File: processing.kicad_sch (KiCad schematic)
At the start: 29 parts, among them U2 DLF162500LT-5028A1, U6 STM32WB35C_C-E_UxA, Y1 32MHz, Y2 32kHz

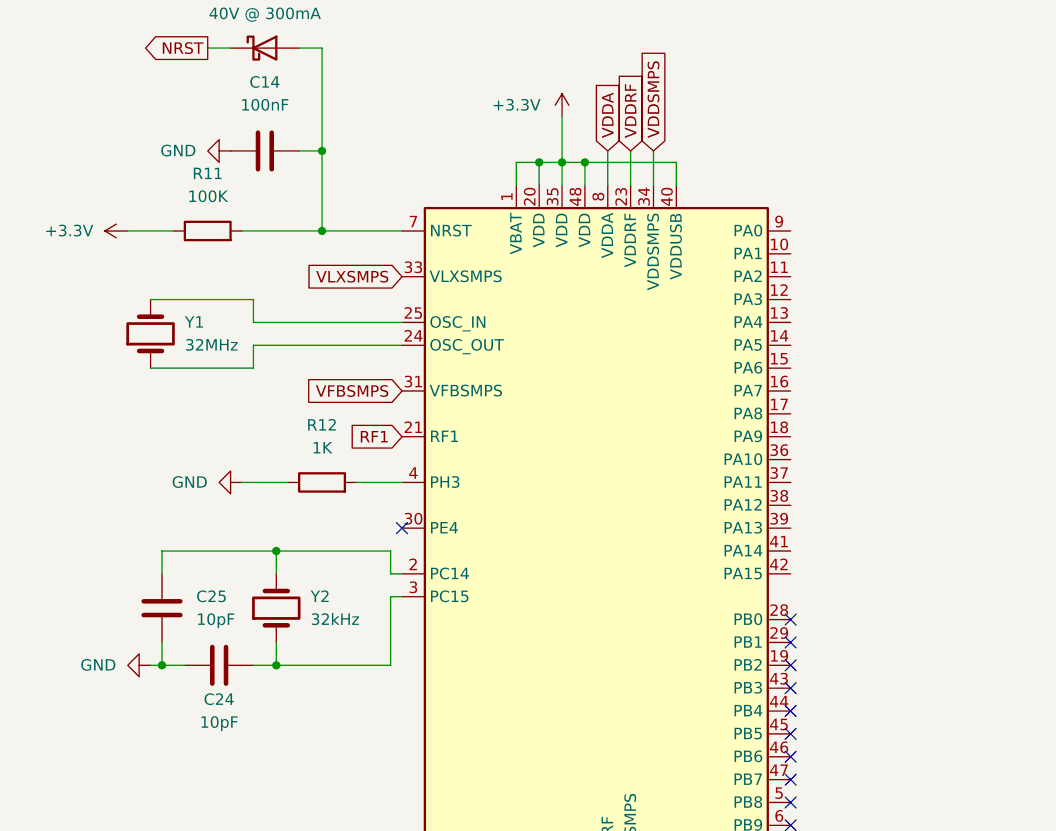
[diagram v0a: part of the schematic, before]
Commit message: Catalogued in raja.rocks
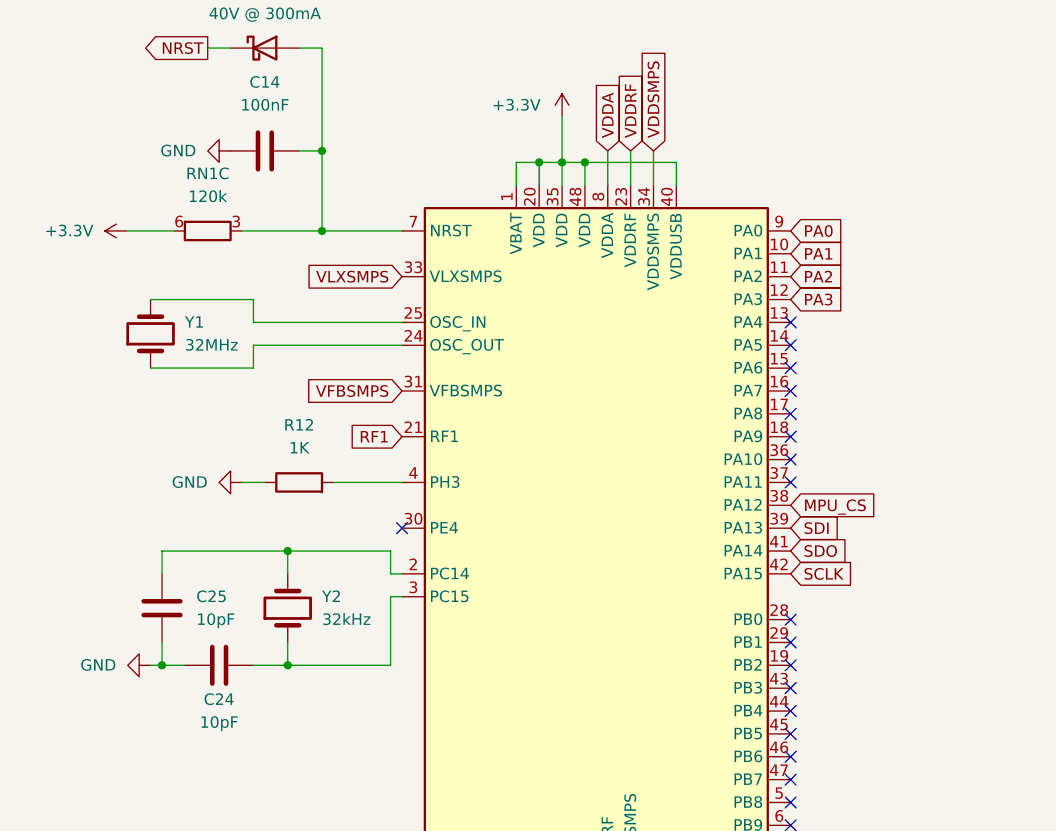
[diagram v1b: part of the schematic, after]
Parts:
- removed R11: 100K, symbol Device:R
- added RN1: 120k, Resistor_SMD:R_Array_Convex_4x1206, symbol Device:R_Pack04_Split
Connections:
- net +3.3V: now also RN1.6 (R3.2)
- net at C14.2, D4.2 (A), U6.7 (NRST): now also RN1.3 (R3.1)
- net PA1: now reaches U6.10 (PA1)
- net PA2: now reaches U6.11 (PA2)
- net PA3: now reaches U6.12 (PA3)
- net MPU_CS: now reaches U6.38 (PA12)
- net SDI: now reaches U6.39 (PA13)
- net SDO: now reaches U6.41 (PA14)
- net SCLK: now reaches U6.42 (PA15)
- net PA0: now reaches U6.9 (PA0)
- no-connect marks 11 -> 19
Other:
- moved on the sheet: R12, Y2
